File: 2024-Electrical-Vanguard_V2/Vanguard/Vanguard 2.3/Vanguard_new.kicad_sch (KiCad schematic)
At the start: 86 parts, among them J1 USB_C_Receptacle_USB2.0_16P, J2 Conn_02x03_Pin, J3 Micro_SD_Card_Det1, J4 STARBOARD_SERVO, J5 PORTSIDE_SERVO, J6 Battery In, J7 EJECTION_SERVO, Q1 BSS138, Q2 BSS138, Q3 BSS138, Q4 BSS138, U1 ATSAMD11D14A-M, U2 ATmega4809-A, U3 AT25DF641A-SH-T, U4 AP2112K-3.3, U5 BD1020HFV, U6 BNO086, U7 TXB0104D, U8 TPS61092, U9 MPM3610AGQV-P, Y1 32.768kHz

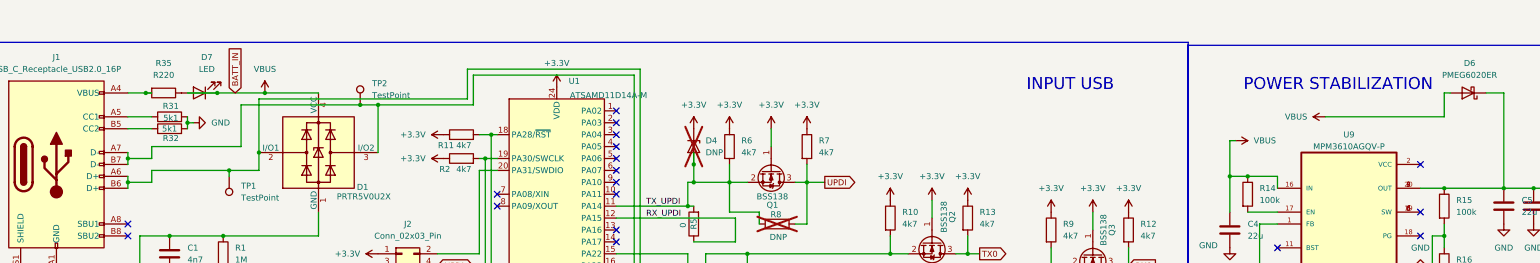
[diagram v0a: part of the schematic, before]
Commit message: fixed the errors in v2.3
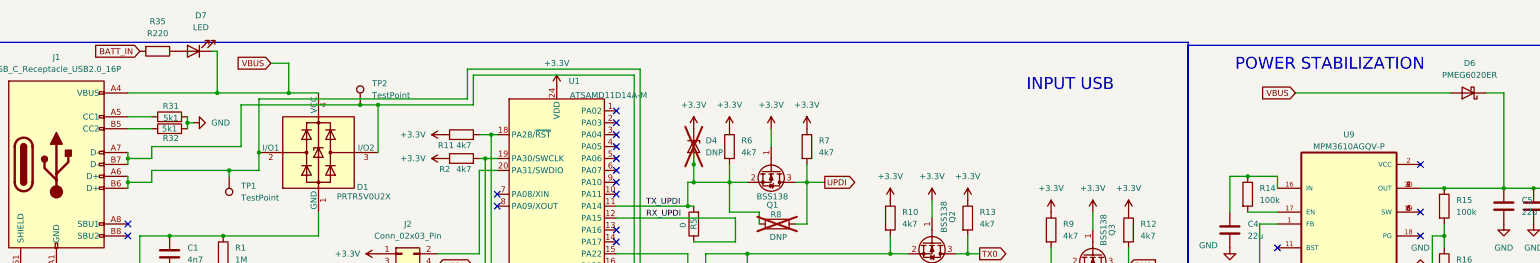
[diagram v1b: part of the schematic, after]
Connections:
- net VBUS: now also J1.A4 (VBUS), J1.A9 (VBUS), J1.B4 (VBUS), J1.B9 (VBUS); no longer C4.1, C8.1, J6.1 (Pin_1), R14.1, R33.2, U8.11 (EN), U8.8 (VBAT), U9.16 (IN)
- new net: C4.1, R14.1, U9.16 (IN)
- new net BATT_IN: C8.1, J6.1 (Pin_1), R33.2, R35.2, U8.11 (EN), U8.8 (VBAT)
